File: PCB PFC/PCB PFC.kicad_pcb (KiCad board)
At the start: 2 copper layers, 45 parts, among them J1 INA_1, J2 INA_2, J4 External_Power, J5 BAT54S_1, J6 BAT54S_2, SW2 SW_Push, U2 L7805, U3 TL082, U4 TL084, U5 TL082, U8 ESP32-C3_SUPERMINI_TH

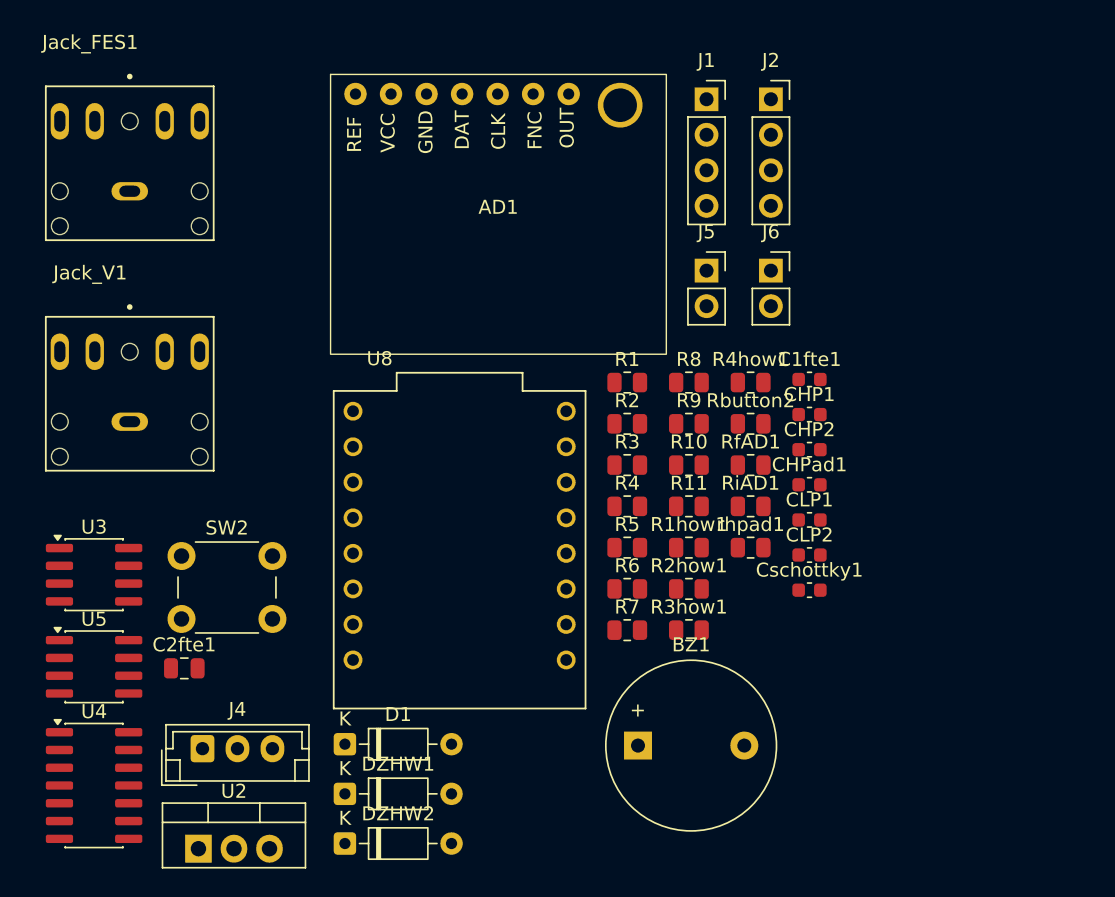
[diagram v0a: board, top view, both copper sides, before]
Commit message: Placa final chidori 3V3 by Gus
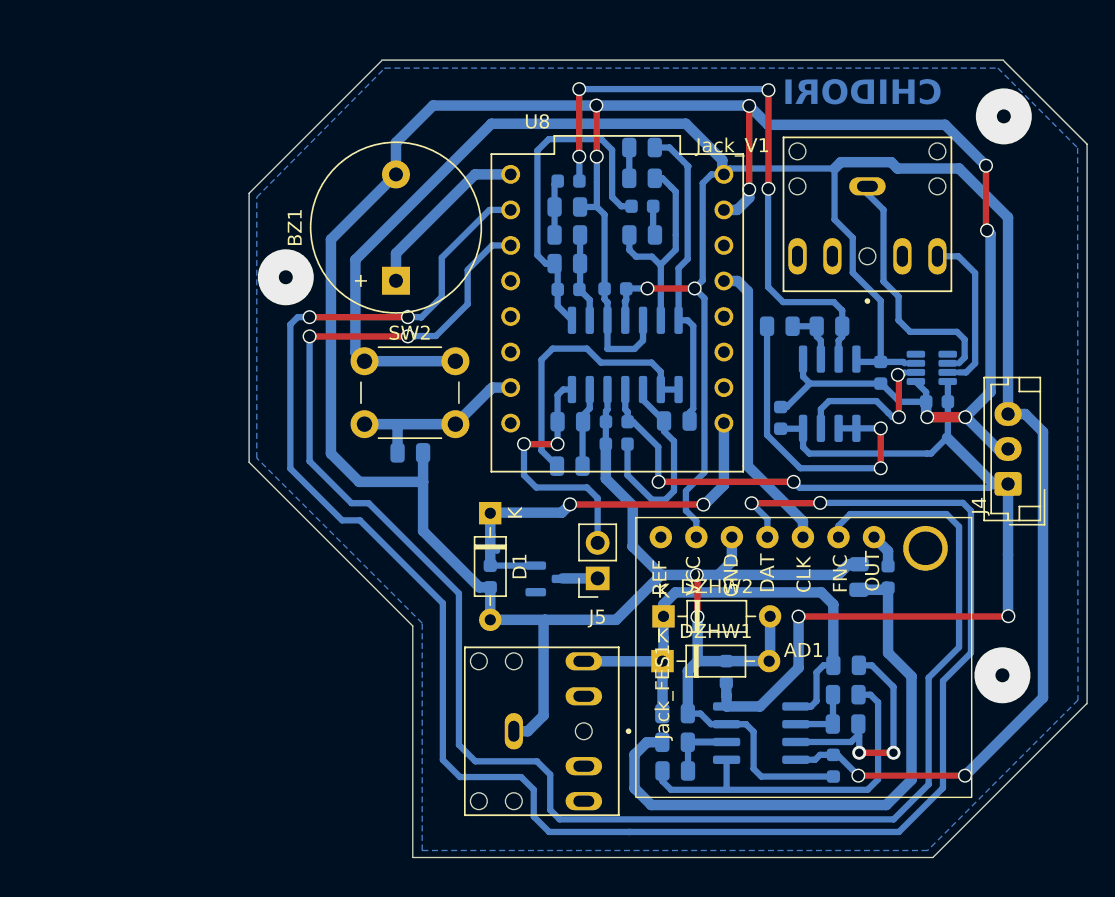
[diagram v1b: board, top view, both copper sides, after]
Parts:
- removed C1fte1: 20pF, Capacitor_SMD:C_0603_1608Metric
- removed C2fte1: 10uFx16V, Capacitor_SMD:C_0805_2012Metric
- removed J1: INA_1, Connector_PinSocket_2.54mm:PinSocket_1x04_P2.54mm_Vertical
- removed J2: INA_2, Connector_PinSocket_2.54mm:PinSocket_1x04_P2.54mm_Vertical
- removed J6: BAT54S_2, Connector_PinSocket_2.54mm:PinSocket_1x02_P2.54mm_Vertical
- removed U2: L7805, Package_TO_SOT_THT:TO-220-3_Vertical
- added Cd_01: 22n, Capacitor_SMD:C_0603_1608Metric, B.Cu at (144.3, 76.3)
- added Cd_2: 22n, Capacitor_SMD:C_0603_1608Metric, B.Cu at (144.4, 85.8)
- added Cd_4: 22n, Capacitor_SMD:C_0603_1608Metric, B.Cu at (156.1, 85.6)
- added Cd_5: 22n, Capacitor_SMD:C_0603_1608Metric, B.Cu at (167.3, 84.4)
- added Cd_6: 22n, Capacitor_SMD:C_0603_1608Metric, B.Cu at (163.2, 82.3)
- added Cd_7: 22n, Capacitor_SMD:C_0603_1608Metric, B.Cu at (159.9, 110.4)
- added Cd_8: 22n, Capacitor_SMD:C_0603_1608Metric, B.Cu at (152.2, 103.7)
- added D2: BAT54S, Package_TO_SOT_SMD:SOT-23, B.Cu at (139.5, 97.1)
- added U1: INA128, Package_TO_SOT_SMD:SOT-23-8, B.Cu at (166.9, 82.0)
- CHP1, CHP2, CHPad1, CLP1, CLP2, Cschottky1, R1, R10, R11, R1how1, R2, R2how1, R3, R3how1, R4, R4how1, R5, R6, R7, R8, R9, Rbutton2, RfAD1, RiAD1, U3, U4, U5, rhpad1: moved to B.Cu
- J5: value BAT54S_1 -> JUMPER_BAT54S
- moved J4 60.6 mm to (172.3, 90.3), turned to 90 degrees
- moved U5 56.1 mm to (159.6, 83.8), turned to 90 degrees
- moved Jack_V1 55.3 mm to (162.3, 69.0), turned to 180 degrees
- moved U3 49.0 mm to (154.7, 108.1)
- moved U4 48.9 mm to (145.0, 81.1), turned to -90 degrees
- moved Jack_FES1 47.4 mm to (137.0, 108.0), turned to -90 degrees
- moved AD1 38.5 mm to (157.8, 102.7)
- moved BZ1 37.5 mm to (128.6, 75.8), turned to 90 degrees
- moved R7 32.3 mm to (146.2, 68.5), turned to 180 degrees
- moved DZHW2 28.0 mm to (147.7, 99.8)
- moved R11 25.9 mm to (146.2, 66.2)
- moved R6 25.3 mm to (146.2, 72.5)
- moved DZHW1 24.6 mm to (147.7, 103.0)
- moved Rbutton2 24.4 mm to (129.6, 88.1)
- moved CHP1 24.0 mm to (140.9, 68.7), turned to 180 degrees
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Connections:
- net /Fes Out+ renamed /FesOut+
- AD1 pad 2: /3v3 -> /+
- J5 pad 1: unconnected-(J5-Pin_1-Pad1) -> /CON_BAT54S
- J5 pad 2: unconnected-(J5-Pin_2-Pad2) -> /SIN_BAT54S
- R10 pad 2: Net-(R10-Pad2) -> /SIN_BAT54S
- SW2 pad 1: /3v3 -> /+
- U4 pad 14: Net-(R10-Pad2) -> /SIN_BAT54S
- U8 pad 2: /alarm -> unconnected-(U8-GPIO2-Pad2)
- U8 pad 3.3: /3v3 -> unconnected-(U8-3V3-Pad3.3)
- U8 pad 5: unconnected-(U8-GPIO5-Pad5) -> /alarm
- U8 pad 5V: /5V -> /+
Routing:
- net GNDREF: track 0.00 -> 252.4 mm, vias 0 -> 10
- net /+: track 0.00 -> 180.0 mm, vias 0 -> 4
- net /data: track 0.00 -> 137.4 mm, vias 0 -> 4
- net /fnc: track 0.00 -> 120.6 mm, vias 0 -> 2
- net /-: track 0.00 -> 91.8 mm, vias 0 -> 4
- net Net-(CHP1-Pad1): track 0.00 -> 43.8 mm, vias 0 -> 4
- net /outAD: track 0.00 -> 42.7 mm
- net /FesOut+: track 0.00 -> 35.8 mm
- net /Vout: track 0.00 -> 29.0 mm, vias 0 -> 2
- net Net-(R1how1-Pad1): track 0.00 -> 26.0 mm
- net Net-(CHP2-Pad1): track 0.00 -> 24.6 mm
- net Net-(U5A--): track 0.00 -> 22.7 mm, vias 0 -> 2
- net Net-(R11-Pad2): track 0.00 -> 22.4 mm
- net /clk: track 0.00 -> 21.2 mm
- net Net-(U4C--): track 0.00 -> 20.1 mm
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- added copper zone on B.Cu, net (none)
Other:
- board outline added: 59.9 x 57 mm
- board text added: "CHIDORI"
